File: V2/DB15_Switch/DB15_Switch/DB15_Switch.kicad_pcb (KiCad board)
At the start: 2 copper layers, 31.7 x 43.7 mm, 35 parts, among them J1 DB15_Male_HighDensity_Mountin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, U1 CH340C, U2 SM420561N, U3 STI3508, U4 ATmega328P-A, Y1 Crystal_GND24

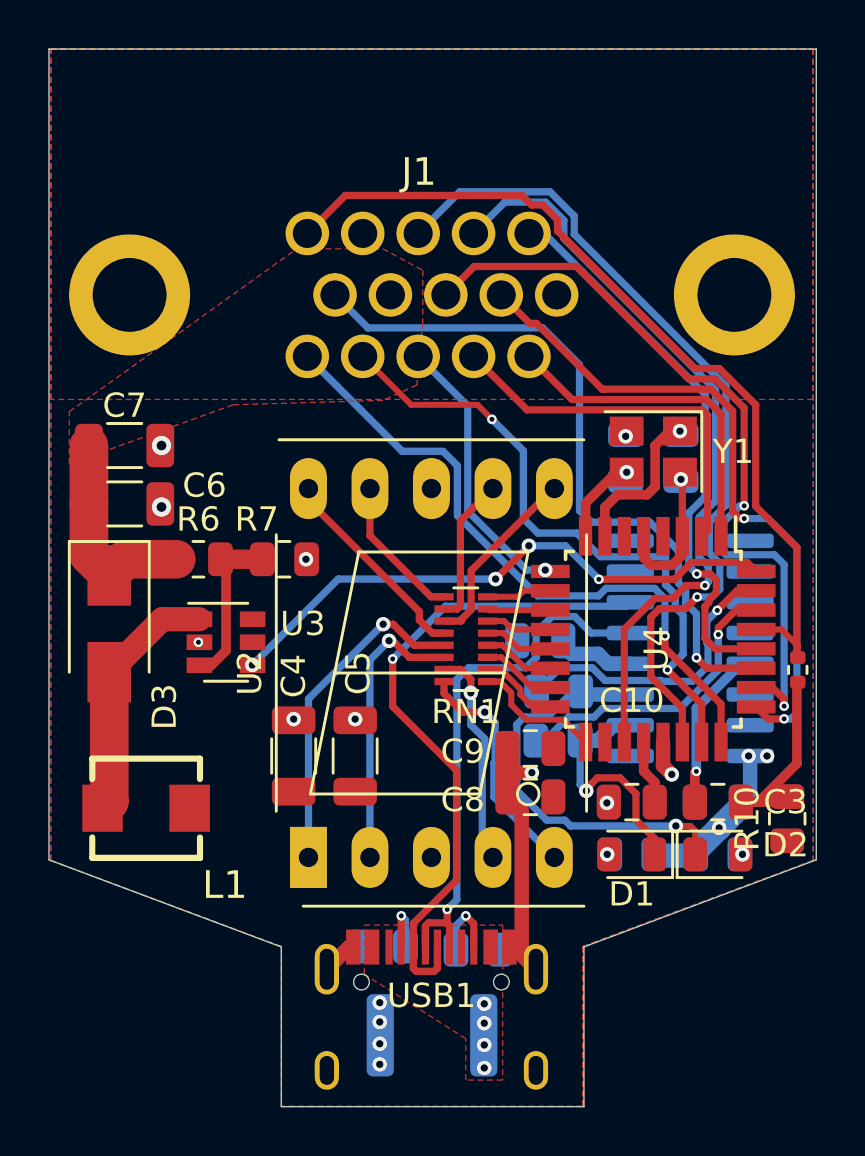
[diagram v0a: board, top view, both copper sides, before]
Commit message: update
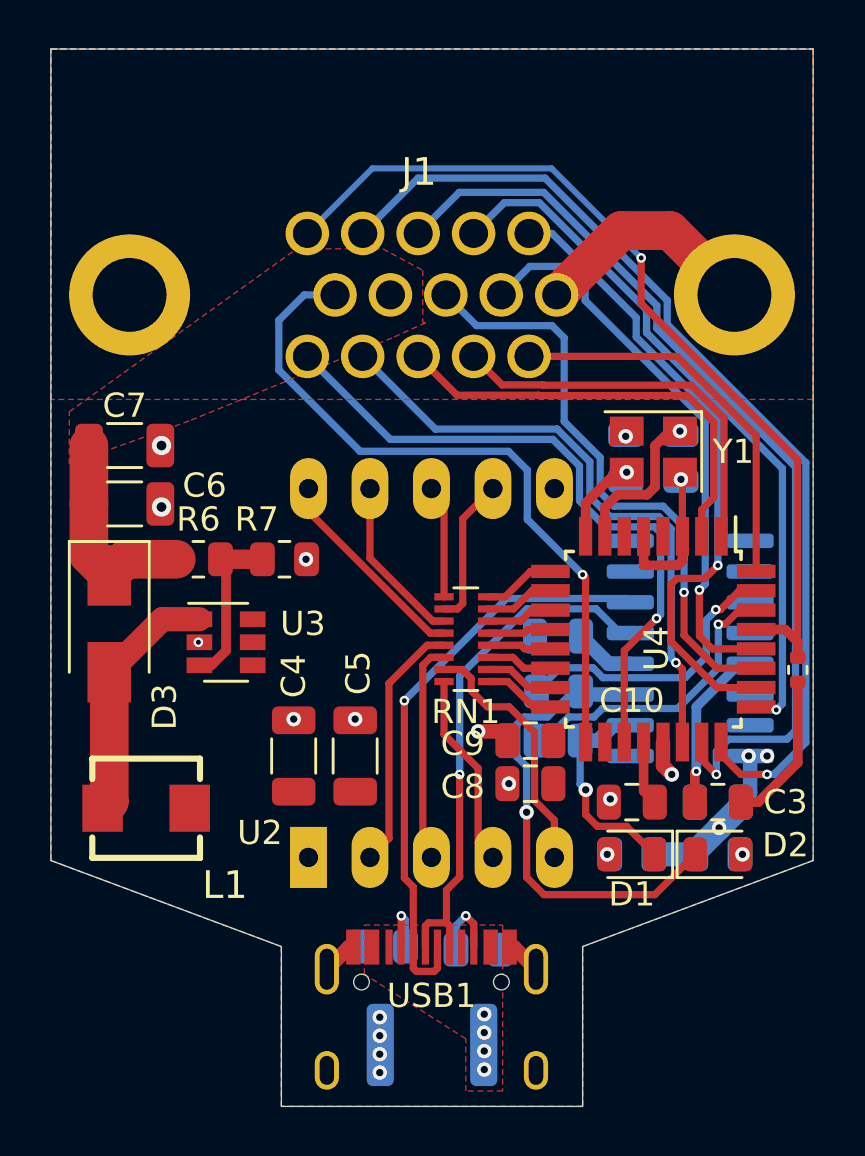
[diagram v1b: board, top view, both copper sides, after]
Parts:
- removed R10: 10K, Resistor_SMD:R_0805_2012Metric
- U2: value SM420561N -> HDSP-A151
- moved C1 0.76 mm to (82.9, 75.1)
- moved C8 0.55 mm to (81.8, 81.2)
- moved F1 0.40 mm to (77.7, 91.9)
- moved C9 0.33 mm to (81.8, 79.4)
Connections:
- J1 pad 1: /D3 -> /D2
- J1 pad 10: /A4 -> /D13
- J1 pad 11: /A5 -> /A3
- J1 pad 12: /A6 -> /A2
- J1 pad 13: /A7 -> /A0
- J1 pad 14: Net-(J1-Pad14) -> /A1
- J1 pad 2: /D4 -> /D3
- J1 pad 3: /D5 -> /D4
- J1 pad 4: /A0 -> /A7
- J1 pad 5: /A1 -> /A6
- J1 pad 7: /A2 -> /A5
- J1 pad 8: /A3 -> /A4
- RN1 pad 1: /D13 -> /D12
- RN1 pad 2: /D12 -> /D11
- RN1 pad 3: /D11 -> /D10
- RN1 pad 4: /D10 -> /D9
- RN1 pad 5: /D9 -> /D8
- RN1 pad 6: /D8 -> /D7
- RN1 pad 7: /D7 -> /D6
- RN1 pad 8: /D6 -> /D5
- U2 pad 1: Net-(RN1-Pad13) -> +5V
- U2 pad 2: Net-(RN1-Pad14) -> Net-(RN1-Pad13)
- U2 pad 3: +5V -> Net-(RN1-Pad14)
- U2 pad 4: Net-(RN1-Pad15) -> Net-(RN1-Pad16)
- U2 pad 5: Net-(RN1-Pad16) -> Net-(RN1-Pad15)
- U2 pad 6: Net-(RN1-Pad11) -> +5V
- U2 pad 8: +5V -> Net-(RN1-Pad9)
- U2 pad 9: Net-(RN1-Pad9) -> Net-(RN1-Pad11)
- U3 pad 4: /D2 -> +5V
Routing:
- net /D13: track 5.37 -> 29.0 mm, vias 0 -> 1
- net /A1: track 27.3 -> 41.2 mm
- net /A0: track 26.4 -> 38.6 mm, vias 2 -> 1
- net /A7: track 35.1 -> 25.5 mm
- net /D5: track 11.7 -> 3.03 mm, vias 1 -> 0
- net /D2: track 23.9 -> 16.4 mm, vias 4 -> 0
- net /A3: track 32.0 -> 26.4 mm, vias 2 -> 1
- net /A4: track 29.5 -> 24.7 mm
- net /A6: track 31.5 -> 27.7 mm
- net Net-(RN1-Pad13): track 13.8 -> 10.4 mm, vias 1 -> 0
- net Net-(U1-Pad6): track 27.4 -> 24.3 mm
- net Net-(RN1-Pad14): track 11.8 -> 9.10 mm, vias 1 -> 0
- net /TX: track 17.1 -> 19.7 mm
- net /D4: track 15.8 -> 18.3 mm
- net /D3: track 14.0 -> 16.3 mm
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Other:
- board size 31.7 x 43.7 mm -> 31.5 x 43.7 mm
